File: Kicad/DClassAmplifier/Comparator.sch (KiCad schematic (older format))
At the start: 5 parts, among them J2 Conn_01x03, U1 LM319

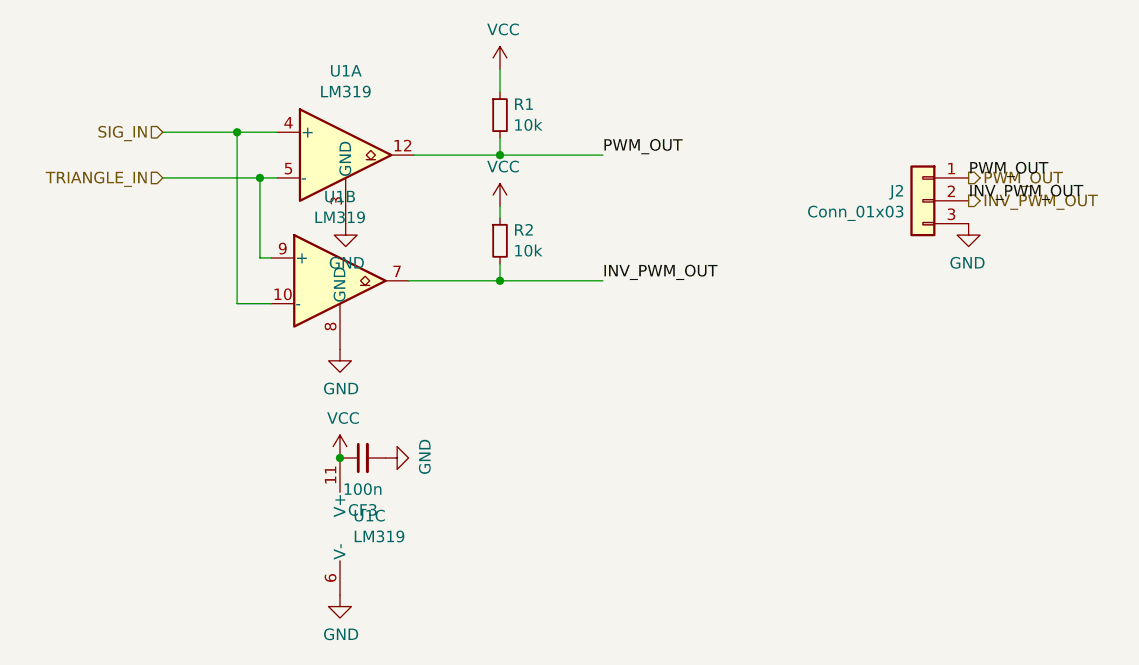
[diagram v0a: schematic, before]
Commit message: Combined Board
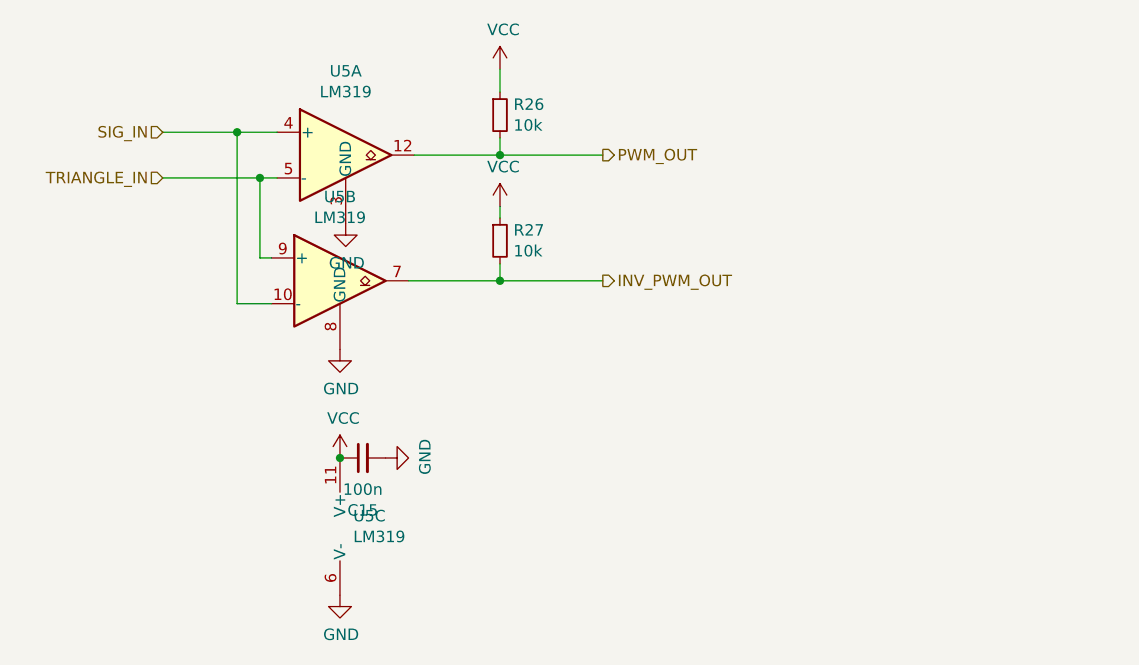
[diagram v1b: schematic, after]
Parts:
- removed J2: Conn_01x03, TerminalBlock:TerminalBlock_bornier-3_P5.08mm, symbol Connector_Generic:Conn_01x03
- C15: renamed from CF3; footprint Capacitor_SMD:C_0805_2012Metric_Pad1.18x1.45mm_HandSolder -> Capacitor_SMD:C_0603_1608Metric_Pad1.08x0.95mm_HandSolder
- renumbered R1 to R26, R2 to R27, U1 to U5
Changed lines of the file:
@@
 $EndDescr
 $Comp
-L Comparator:LM319 U1
+L Comparator:LM319 U5
 U 1 1 61116116
 P 5150 2875
-F 0 "U1" H 5150 3242 50  0000 C CNN
+F 0 "U5" H 5150 3242 50  0000 C CNN
 F 1 "LM319" H 5150 3151 50  0000 C CNN
 F 2 "Package_SO:SO-14_3.9x8.65mm_P1.27mm" H 5150 2875 50  0001 C CNN
@@
 $EndComp
 $Comp
-L Comparator:LM319 U1
+L Comparator:LM319 U5
 U 2 1 6111611C
 P 5125 3425
-F 0 "U1" H 5125 3792 50  0000 C CNN
+F 0 "U5" H 5125 3792 50  0000 C CNN
 F 1 "LM319" H 5125 3701 50  0000 C CNN
 F 2 "Package_SO:SO-14_3.9x8.65mm_P1.27mm" H 5125 3425 50  0001 C CNN
@@
 $EndComp
 $Comp
-L Comparator:LM319 U1
+L Comparator:LM319 U5
 U 3 1 61116122
 P 5225 4500
-F 0 "U1" H 5183 4546 50  0000 L CNN
+F 0 "U5" H 5183 4546 50  0000 L CNN
 F 1 "LM319" H 5183 4455 50  0000 L CNN
 F 2 "Package_SO:SO-14_3.9x8.65mm_P1.27mm" H 5225 4500 50  0001 C CNN
@@
 	4675 3525 4825 3525
 $Comp
-L power:GND #PWR010
+L power:GND #PWR044
 U 1 1 61116132
 P 5150 3175
-F 0 "#PWR010" H 5150 2925 50  0001 C CNN
+F 0 "#PWR044" H 5150 2925 50  0001 C CNN
 F 1 "GND" H 5155 3002 50  0000 C CNN
 F 2 "" H 5150 3175 50  0001 C CNN
@@
 $EndComp
 $Comp
-L power:GND #PWR07
+L power:GND #PWR045
 U 1 1 61116138
 P 5125 3725
-F 0 "#PWR07" H 5125 3475 50  0001 C CNN
+F 0 "#PWR045" H 5125 3475 50  0001 C CNN
 F 1 "GND" H 5130 3552 50  0000 C CNN
 F 2 "" H 5125 3725 50  0001 C CNN
@@
 $EndComp
 $Comp
-L power:GND #PWR09
+L power:GND #PWR048
 U 1 1 6111613E
 P 5125 4800
-F 0 "#PWR09" H 5125 4550 50  0001 C CNN
+F 0 "#PWR048" H 5125 4550 50  0001 C CNN
 F 1 "GND" H 5130 4627 50  0000 C CNN
 F 2 "" H 5125 4800 50  0001 C CNN
@@
 $EndComp
 $Comp
-L power:VCC #PWR08
+L power:VCC #PWR046
 U 1 1 61116144
 P 5125 4200
-F 0 "#PWR08" H 5125 4050 50  0001 C CNN
+F 0 "#PWR046" H 5125 4050 50  0001 C CNN
 F 1 "VCC" H 5140 4373 50  0000 C CNN
 F 2 "" H 5125 4200 50  0001 C CNN
@@
 	1    0    0    -1
 $EndComp
-Text HLabel 7875 3075 2    50   Output ~ 0
-INV_PWM_OUT
 Text HLabel 4350 2975 0    50   Input ~ 0
 TRIANGLE_IN
@@
 	5425 3425 5825 3425
 $Comp
-L Device:R_Small R1
+L Device:R_Small R26
 U 1 1 61119BD5
 P 5825 2700
-F 0 "R1" H 5884 2746 50  0000 L CNN
+F 0 "R26" H 5884 2746 50  0000 L CNN
 F 1 "10k" H 5884 2655 50  0000 L CNN
 F 2 "Resistor_SMD:R_0603_1608Metric_Pad0.98x0.95mm_HandSolder" H 5825 2700 50  0001 C CNN
@@
 $EndComp
 $Comp
-L Device:R_Small R2
+L Device:R_Small R27
 U 1 1 6111A188
 P 5825 3250
-F 0 "R2" H 5884 3296 50  0000 L CNN
+F 0 "R27" H 5884 3296 50  0000 L CNN
 F 1 "10k" H 5884 3205 50  0000 L CNN
 F 2 "Resistor_SMD:R_0603_1608Metric_Pad0.98x0.95mm_HandSolder" H 5825 3250 50  0001 C CNN
@@
 $EndComp
 $Comp
-L power:VCC #PWR011
+L power:VCC #PWR042
 U 1 1 6111A8CA
 P 5825 2500
-F 0 "#PWR011" H 5825 2350 50  0001 C CNN
+F 0 "#PWR042" H 5825 2350 50  0001 C CNN
 F 1 "VCC" H 5840 2673 50  0000 C CNN
 F 2 "" H 5825 2500 50  0001 C CNN
@@
 $EndComp
 $Comp
-L power:VCC #PWR012
+L power:VCC #PWR043
 U 1 1 6111AE94
 P 5825 3100
-F 0 "#PWR012" H 5825 2950 50  0001 C CNN
+F 0 "#PWR043" H 5825 2950 50  0001 C CNN
 F 1 "VCC" H 5840 3273 50  0000 C CNN
 F 2 "" H 5825 3100 50  0001 C CNN
@@
 	4775 2975 4350 2975
 Connection ~ 4775 2975
-$Comp
-L Connector_Generic:Conn_01x03 J2
-U 1 1 611080B2
-P 7675 3075
-F 0 "J2" H 7755 3117 50  0000 L CNN
-F 1 "Conn_01x03" H 7755 3026 50  0000 L CNN
-F 2 "TerminalBlock:TerminalBlock_bornier-3_P5.08mm" H 7675 3075 50  0001 C CNN
-F 3 "~" H 7675 3075 50  0001 C CNN
-	1    7675 3075
-	-1   0    0    -1
-$EndComp
-Text HLabel 7875 2975 2    50   Output ~ 0
-PWM_OUT
 Connection ~ 5825 2875
 Wire Wire Line
 	6275 2875 5825 2875
 $Comp
-L power:GND #PWR013
-U 1 1 6110885B
-P 7875 3175
-F 0 "#PWR013" H 7875 2925 50  0001 C CNN
-F 1 "GND" H 7880 3002 50  0000 C CNN
-F 2 "" H 7875 3175 50  0001 C CNN
-F 3 "" H 7875 3175 50  0001 C CNN
-	1    7875 3175
-	-1   0    0    -1
-$EndComp
-Text Label 7875 2975 0    50   ~ 0
-PWM_OUT
-Text Label 7875 3075 0    50   ~ 0
-INV_PWM_OUT
-Text Label 6275 2875 0    50   ~ 0
-PWM_OUT
-Text Label 6275 3425 0    50   ~ 0
-INV_PWM_OUT
-$Comp
-L Device:C_Small CF?
+L Device:C_Small C?
 U 1 1 611DC342
 P 5225 4200
-AR Path="/610C616D/611DC342" Ref="CF?"  Part="1"
-AR Path="/611D4178/611DC342" Ref="CF?"  Part="1"
-AR Path="/61113C55/611DC342" Ref="CF3"  Part="1"
-F 0 "CF3" V 4996 4200 50  0000 C CNN
+AR Path="/610C616D/611DC342" Ref="C?"  Part="1"
+AR Path="/611D4178/611DC342" Ref="C?"  Part="1"
+AR Path="/61113C55/611DC342" Ref="C15"  Part="1"
+F 0 "C15" V 4996 4200 50  0000 C CNN
 F 1 "100n" V 5087 4200 50  0000 C CNN
-F 2 "Capacitor_SMD:C_0805_2012Metric_Pad1.18x1.45mm_HandSolder" H 5225 4200 50  0001 C CNN
+F 2 "Capacitor_SMD:C_0603_1608Metric_Pad1.08x0.95mm_HandSolder" H 5225 4200 50  0001 C CNN
 F 3 "~" H 5225 4200 50  0001 C CNN
 	1    5225 4200
@@
 $EndComp
 $Comp
-L power:GND #PWR?
+L power:GND #PWR047
 U 1 1 611DC348
 P 5325 4200
-F 0 "#PWR?" H 5325 3950 50  0001 C CNN
+F 0 "#PWR047" H 5325 3950 50  0001 C CNN
 F 1 "GND" H 5330 4027 50  0000 C CNN
 F 2 "" H 5325 4200 50  0001 C CNN
@@
 $EndComp
 Connection ~ 5125 4200
+Text HLabel 6275 3425 2    50   Output ~ 0
+INV_PWM_OUT
+Text HLabel 6275 2875 2    50   Output ~ 0
+PWM_OUT
 $EndSCHEMATC
